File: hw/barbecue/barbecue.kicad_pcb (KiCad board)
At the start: 2 copper layers, 124.5 x 54.8 mm, 46 parts, among them J1 47590-0001, J10 TFT, J11 SDCard, J2 Screw_Terminal_01x02, J3 bootsel, J4 gnd clk swd, J5 +pwm3-, J6 R_{ntc}, J7 +pwm3-, J8 +pwm3-, J9 OLED, Q2 AO3400A, Q3 AO3400A, Q4 AO3400A, SW1 EN11-HSM1AF15, U1 W25Q128JVS, U2 RP2040, U3 AMS1117-3.3, Y1 X322512MSB4SI

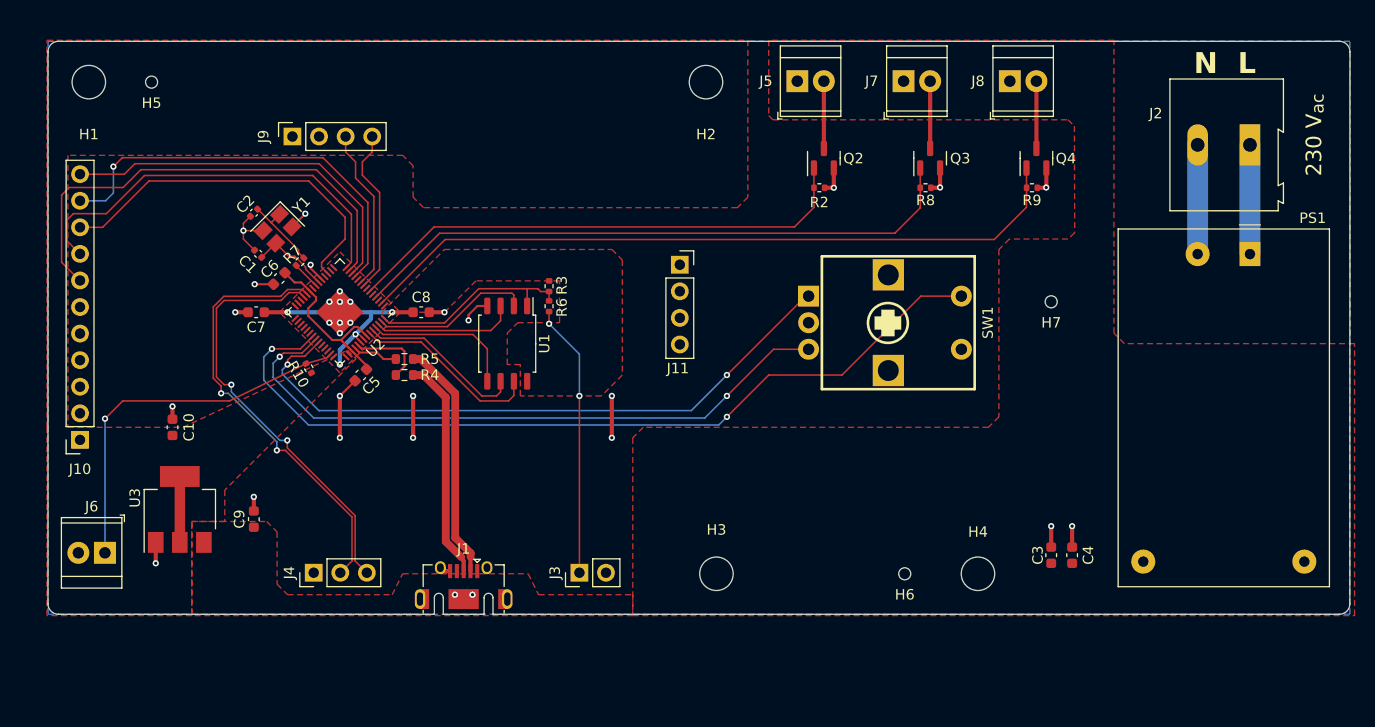
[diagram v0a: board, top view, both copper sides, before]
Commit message: Version 1.1 as sent to manufacturing
Signed-off-by: Jan Hamal Dvořák <mordae@anilinux.org>
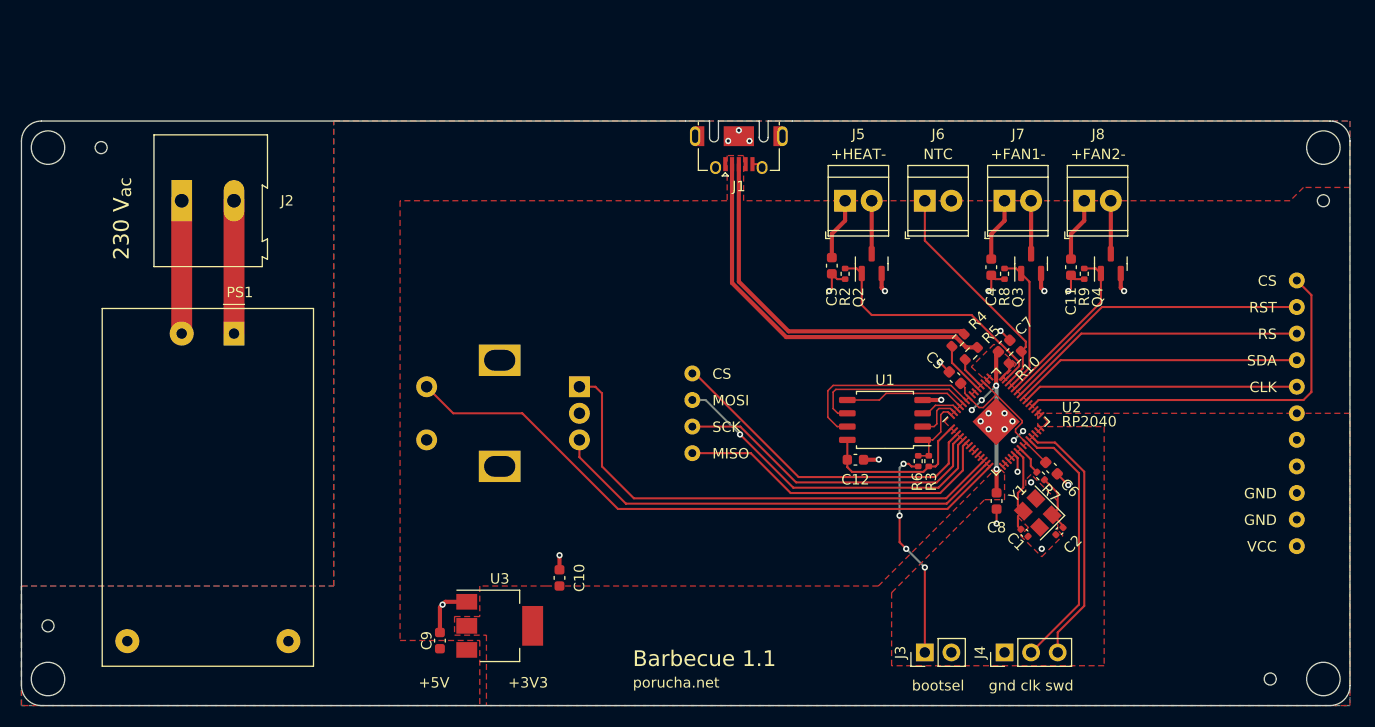
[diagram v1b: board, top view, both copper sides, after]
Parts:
- removed J10: TFT, Connector_PinSocket_2.54mm:PinSocket_1x11_P2.54mm_Vertical
- removed J11: SDCard, Connector_PinSocket_2.54mm:PinSocket_1x04_P2.54mm_Vertical
- removed J9: OLED, Connector_PinSocket_2.54mm:PinSocket_1x04_P2.54mm_Vertical
- added C11: 22u, Capacitor_SMD:C_0603_1608Metric, F.Cu at (135.9, 59.7)
- added C12: 22u, Capacitor_SMD:C_0603_1608Metric, F.Cu at (115.3, 78.1)
- added H8: Tooling, Barbecue:ToolingHole, F.Cu at (160.0, 53.3)
- added U4: ILI9225-MOD, Barbecue:ILI9225-MOD, B.Cu at (129.5, 73.7)
- J5: value +pwm3- -> +HEAT-
- J6: value R_{ntc} -> NTC
- J7: value +pwm3- -> +FAN1-
- J8: value +pwm3- -> +FAN2-
- R10: footprint Resistor_SMD:R_0402_1005Metric -> Resistor_SMD:R_0603_1608Metric
- SW1: moved to B.Cu
- moved PS1 97.4 mm to (55.9, 66.0)
- moved J2 97.3 mm to (50.9, 53.3)
- moved H6 87.0 mm to (43.2, 48.3)
- moved J6 85.3 mm to (121.9, 53.3), turned to 0 degrees
- moved C2 82.8 mm to (134.8, 84.9)
- moved C1 78.0 mm to (131.4, 85.1), turned to 135 degrees
- moved Y1 77.6 mm to (132.7, 83.2), turned to 135 degrees
- moved C6 76.0 mm to (134.0, 78.9), turned to -45 degrees
- moved R7 73.7 mm to (133.0, 79.6), turned to 135 degrees
- moved C7 71.6 mm to (129.5, 67.2), turned to 45 degrees
- moved H3 70.9 mm to (160.0, 48.3)
- moved R10 67.5 mm to (130.6, 68.3), turned to 45 degrees
- moved J4 66.5 mm to (129.5, 96.5)
- moved U2 63.6 mm to (128.7, 74.5), turned to 45 degrees
- moved H2 63.2 mm to (38.1, 48.3)
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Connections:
- Q2 pad 1: /PWM_{3} -> /heat
- Q3 pad 1: /PWM_{2} -> /fan1
- Q4 pad 1: /PWM_{1} -> /fan2
- R2 pad 1: /PWM_{3} -> /heat
- R8 pad 1: /PWM_{2} -> /fan1
- R9 pad 1: /PWM_{1} -> /fan2
- U2 pad 11: /tft_rst -> unconnected-(U2-GPIO8-Pad11)
- U2 pad 12: /tft_cs -> /re_a
- U2 pad 13: /tft_sclk -> /re_b
- U2 pad 14: /tft_mosi -> /re_sw
- U2 pad 17: /tft_rs -> unconnected-(U2-GPIO14-Pad17)
- U2 pad 2: /PWM_{1} -> unconnected-(U2-GPIO0-Pad2)
- U2 pad 3: unconnected-(U2-GPIO1) -> /sd_cs
- U2 pad 32: unconnected-(U2-GPIO21) -> /tft_cs
- U2 pad 34: unconnected-(U2-GPIO22) -> /tft_sck
- U2 pad 35: /re_sw -> /tft_mosi
- U2 pad 36: /re_b -> /tft_rs
- U2 pad 37: /re_a -> /tft_rst
- U2 pad 38: unconnected-(U2-GPIO26_ADC0) -> /fan2
- U2 pad 39: unconnected-(U2-GPIO27_ADC1) -> /fan1
- U2 pad 4: /PWM_{2} -> /sd_sck
- U2 pad 40: unconnected-(U2-GPIO28_ADC2) -> /tsense
- U2 pad 41: /tsense -> /heat
- U2 pad 5: unconnected-(U2-GPIO3) -> /sd_mosi
- U2 pad 6: /PWM_{3} -> /sd_miso
- U2 pad 8: /sda -> unconnected-(U2-GPIO6-Pad8)
- U2 pad 9: /scl -> unconnected-(U2-GPIO7-Pad9)
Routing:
- net /PWM_{1}: track 69.2 -> 0.00 mm
- net /PWM_{2}: track 59.4 -> 0.00 mm
- net /PWM_{3}: track 49.6 -> 0.00 mm
- net /tft_sclk: track 45.8 -> 0.00 mm
- net /sd_mosi: track 0.00 -> 32.6 mm, vias 0 -> 1
- net /sd_cs: track 0.00 -> 32.3 mm
- net /sd_miso: track 0.00 -> 31.1 mm
- net /sd_sck: track 0.00 -> 30.9 mm
- net /tft_sck: track 0.00 -> 26.4 mm
- net /heat: track 0.00 -> 24.4 mm
- net /re_sw: track 81.3 -> 60.4 mm, vias 2 -> 0
- net +5V: track 0.00 -> 18.2 mm
- net /re_b: track 61.9 -> 44.1 mm, vias 2 -> 0
- net /swdclk: track 42.1 -> 25.1 mm, vias 2 -> 0
- net /swdio: track 41.2 -> 24.7 mm, vias 2 -> 0
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- added copper zone on F.Cu, net GND
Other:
- board size 124.5 x 54.8 mm -> 127 x 55.9 mm
- board text added: "+3V3"
- board text added: "+5V"
- board text added: "Barbecue 1.1"
- board text added: "porucha.net"
- board text removed: "L N"
- board text removed: "N L"
